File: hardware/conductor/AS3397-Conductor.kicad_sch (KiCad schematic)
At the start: 37 parts, among them J1 ES, J11 POWER, J2 AudioJack3, J2 MIDI IN, Q1 BS170F, U1 TL072, U4 Teensy-LC, U5 6N138

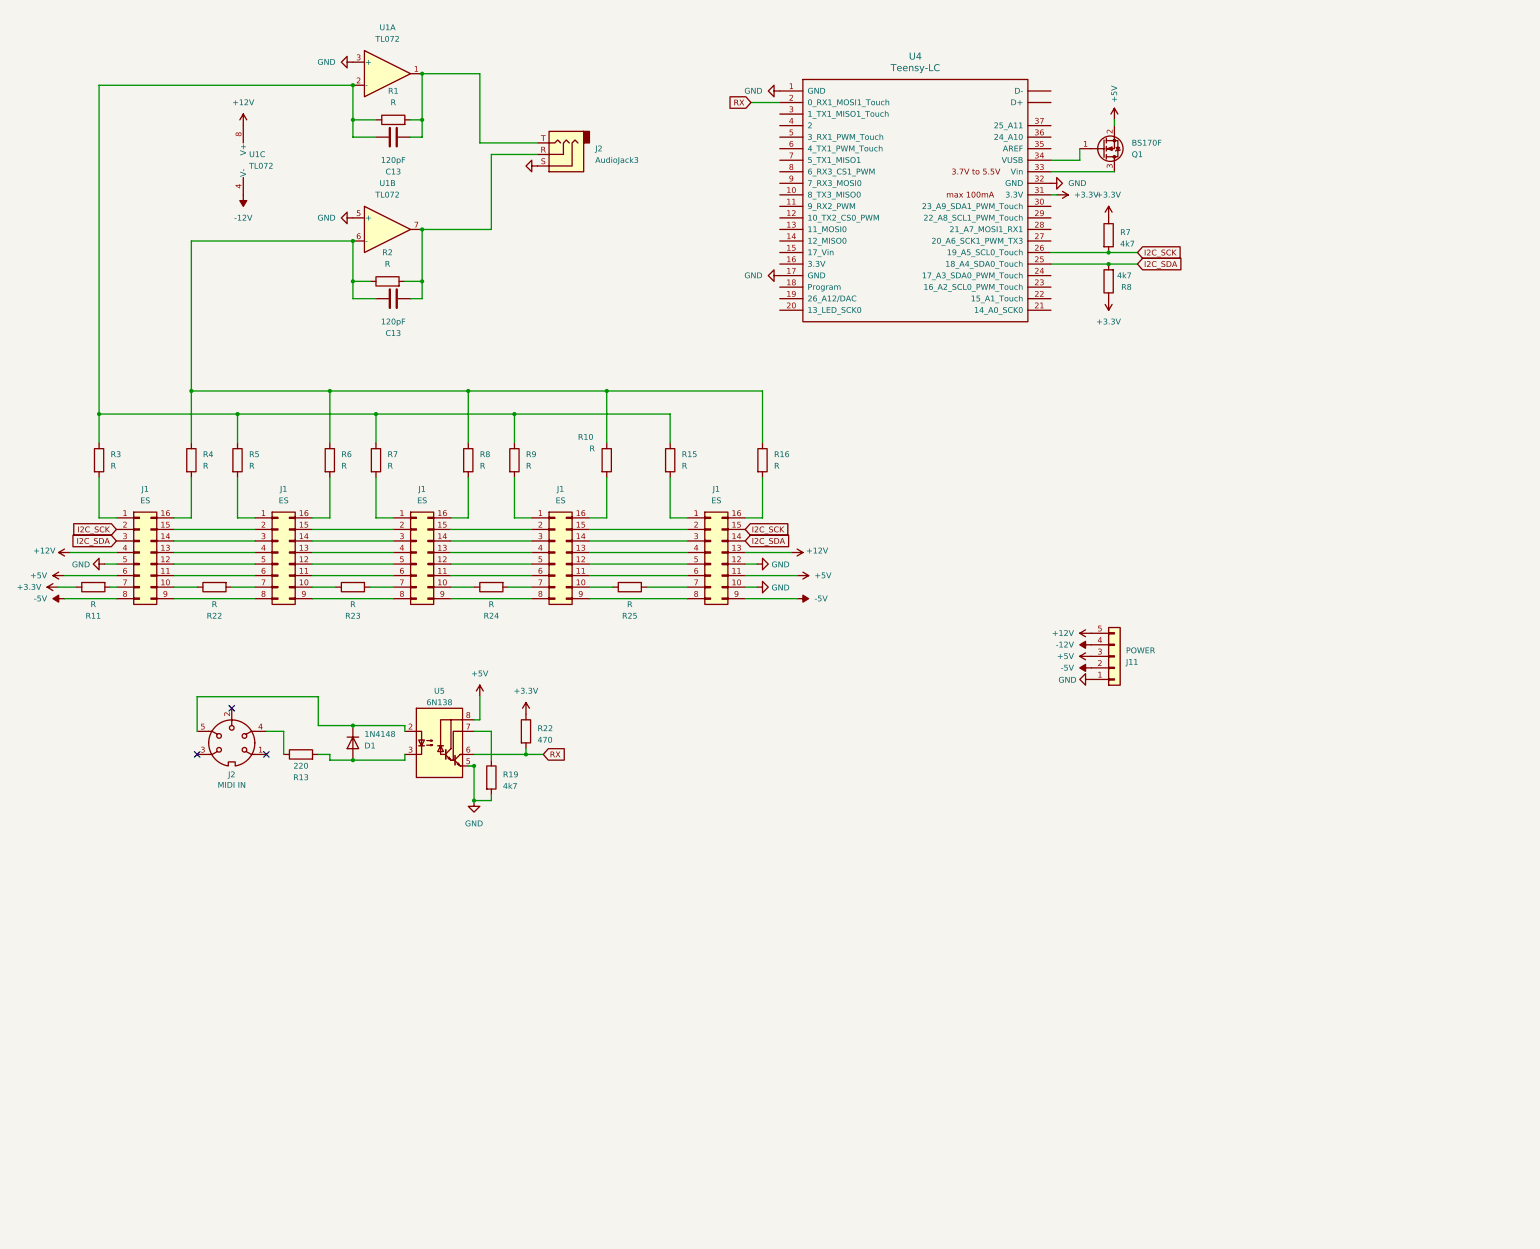
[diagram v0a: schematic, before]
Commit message: Conductor board new version
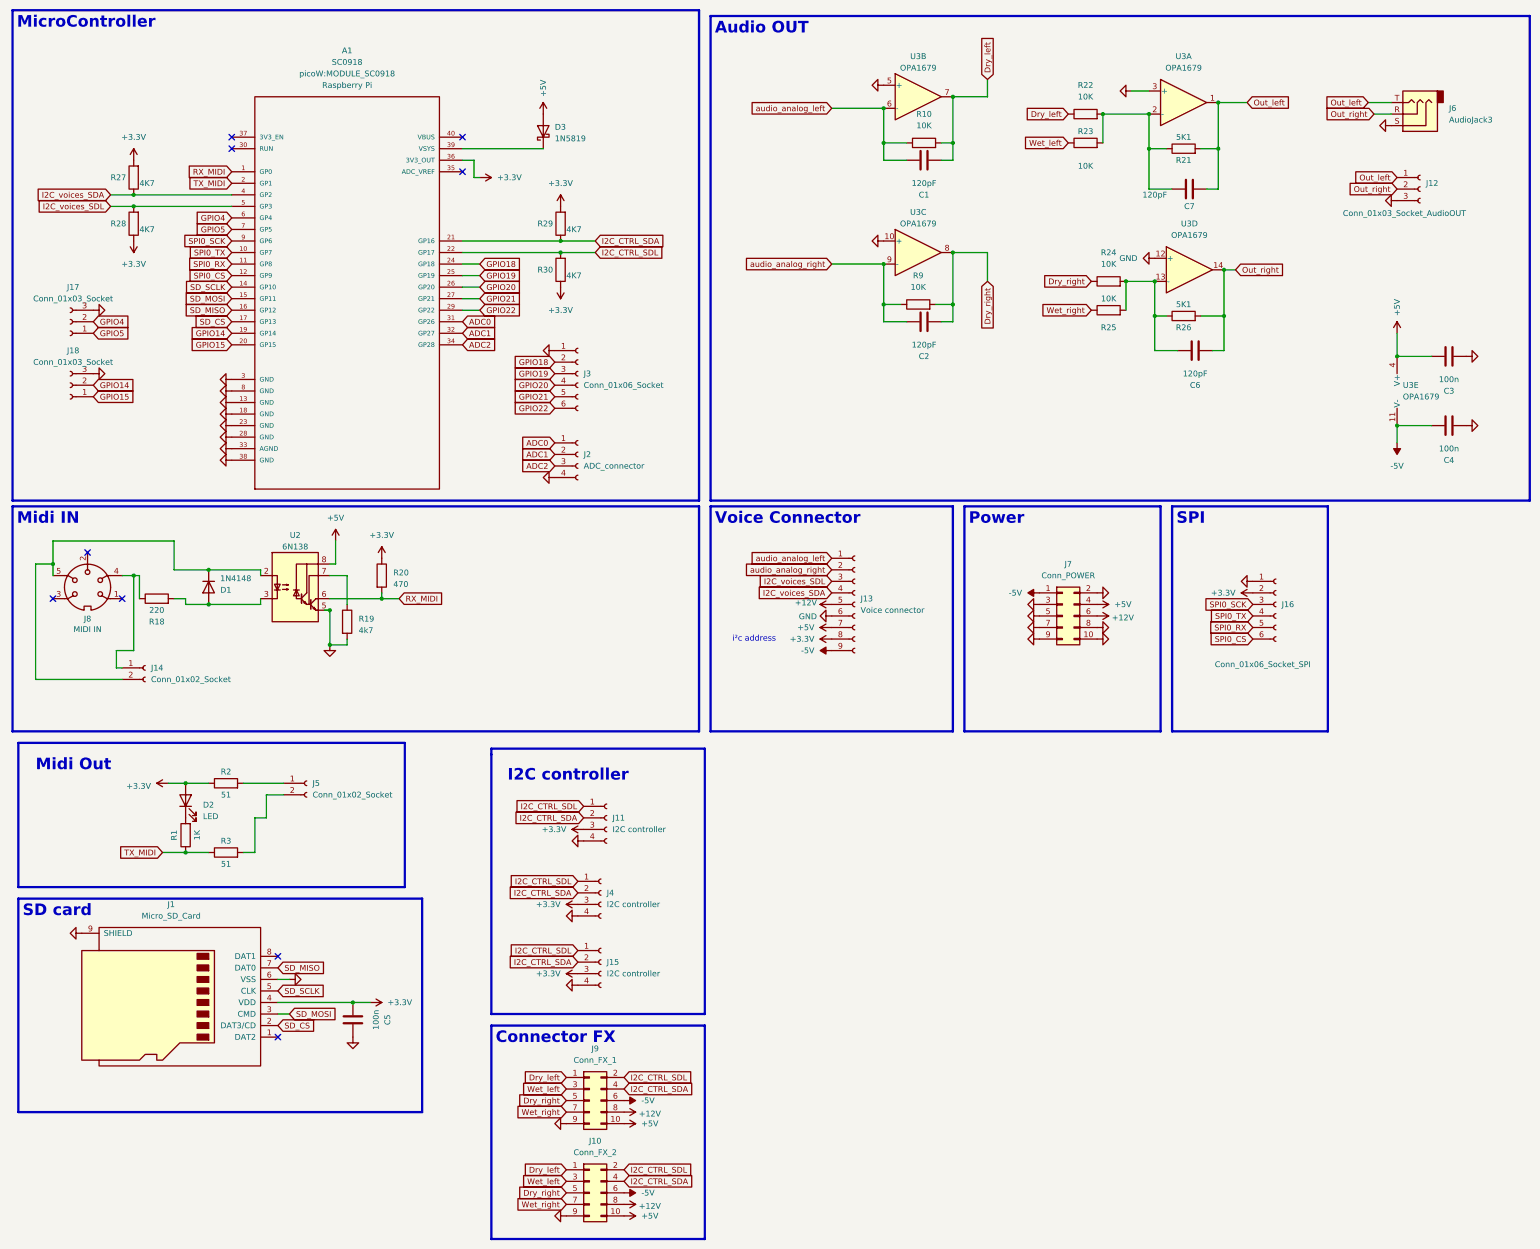
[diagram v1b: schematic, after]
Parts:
- removed C13 (x2): 120pF, Capacitor_THT:C_Disc_D4.3mm_W1.9mm_P5.00mm, symbol Device:C
- removed J1 (x5): ES, SYNTHFILLE:DIP-16_AS, symbol Connector_Generic:Conn_02x08_Counter_Clockwise
- removed J11: POWER, TerminalBlock:TerminalBlock_bornier-4_P5.08mm, symbol Connector_Generic:Conn_01x05
- removed J2: AudioJack3, Connector_Audio:Jack_3.5mm_Ledino_KB3SPRS_Horizontal, symbol Connector_Audio:AudioJack3
- removed J2: MIDI IN, lib:MIDI_DIN5, symbol ES1-rescue:DIN-5-MIDI
- removed Q1: BS170F, Package_TO_SOT_SMD:SOT-23, symbol Transistor_FET:BS170F
- removed R1, R11, R15, R16, R2, R22, R3, R4, R5, R6, R7, R8: R, Resistor_THT:R_Axial_DIN0204_L3.6mm_D1.6mm_P7.62mm_Horizontal, symbol Device:R
- removed R13: 220, Resistor_THT:R_Axial_DIN0204_L3.6mm_D1.6mm_P7.62mm_Horizontal, symbol Device:R
- removed R22: 470, Resistor_THT:R_Axial_DIN0204_L3.6mm_D1.6mm_P7.62mm_Horizontal, symbol Device:R
- removed R7, R8: 4k7, Resistor_THT:R_Axial_DIN0204_L3.6mm_D1.6mm_P7.62mm_Horizontal, symbol Device:R
- removed U1: TL072, Package_DIP:DIP-8_W7.62mm_LongPads, symbol Amplifier_Operational:TL072
- removed U4: Teensy-LC, symbol teensy:Teensy-LC
- removed U5: 6N138, Package_DIP:DIP-8_W7.62mm_LongPads, symbol Isolator:6N138
- added A1: SC0918, picoW:MODULE_SC0918, symbol Raspberry_Pi_Pico_W_SC0918:SC0918
- added C1, C2, C6, C7: 120pF, Capacitor_SMD:C_1206_3216Metric_Pad1.33x1.80mm_HandSolder, symbol Device:C
- added C3, C4, C5: 100n, Capacitor_SMD:C_1206_3216Metric_Pad1.33x1.80mm_HandSolder, symbol Device:C
- added D2: LED, Diode_THT:D_A-405_P2.54mm_Vertical_AnodeUp, symbol Device:LED
- added D3: 1N5819, Diode_THT:D_DO-41_SOD81_P10.16mm_Horizontal, symbol Diode:1N5819
- added J1: Micro_SD_Card, SD_card:J_SD_Card-micro_socket_A, symbol Connector:Micro_SD_Card
- added J10: Conn_FX_2, Connector_PinHeader_2.54mm:PinHeader_2x05_P2.54mm_Vertical, symbol Connector_Generic:Conn_02x05_Odd_Even
- added J11, J15, J4: I2C controller, Connector_JST:JST_EH_B4B-EH-A_1x04_P2.50mm_Vertical, symbol Connector:Conn_01x04_Socket
- added J12: Conn_01x03_Socket_AudioOUT, Connector_JST:JST_EH_B3B-EH-A_1x03_P2.50mm_Vertical, symbol Connector:Conn_01x03_Socket
- added J13: Voice connector, Connector_JST:JST_EH_B9B-EH-A_1x09_P2.50mm_Vertical, symbol Connector:Conn_01x09_Socket
- added J14, J5: Conn_01x02_Socket, Connector_JST:JST_EH_B2B-EH-A_1x02_P2.50mm_Vertical, symbol Connector:Conn_01x02_Socket
- added J16: Conn_01x06_Socket_SPI, Connector_PinSocket_2.54mm:PinSocket_1x06_P2.54mm_Vertical, symbol Connector:Conn_01x06_Socket
- added J17, J18: Conn_01x03_Socket, Connector_PinHeader_2.54mm:PinHeader_1x03_P2.54mm_Vertical, symbol Connector:Conn_01x03_Socket
- added J2: ADC_connector, Connector_JST:JST_EH_B4B-EH-A_1x04_P2.50mm_Vertical, symbol Connector:Conn_01x04_Socket
- added J3: Conn_01x06_Socket, Connector_PinHeader_2.54mm:PinHeader_1x06_P2.54mm_Vertical, symbol Connector:Conn_01x06_Socket
- added J6: AudioJack3, Connector_Audio:Jack_3.5mm_Ledino_KB3SPRS_Horizontal, symbol Connector_Audio:AudioJack3
- added J7: Conn_POWER, Connector_PinHeader_2.54mm:PinHeader_2x05_P2.54mm_Vertical, symbol Connector_Generic:Conn_02x05_Odd_Even
- added J8: MIDI IN, Eurocad:MIDI_DIN5, symbol ES1-rescue:DIN-5-MIDI
- added J9: Conn_FX_1, Connector_PinHeader_2.54mm:PinHeader_2x05_P2.54mm_Vertical, symbol Connector_Generic:Conn_02x05_Odd_Even
- added R1: 1K, Resistor_SMD:R_1206_3216Metric_Pad1.30x1.75mm_HandSolder, symbol Audio_chip:R
- added R18: 220, Resistor_SMD:R_1206_3216Metric_Pad1.30x1.75mm_HandSolder, symbol Device:R
- added R2, R3: 51, Resistor_SMD:R_1206_3216Metric_Pad1.30x1.75mm_HandSolder, symbol Audio_chip:R
- added R20: 470, Resistor_SMD:R_1206_3216Metric_Pad1.30x1.75mm_HandSolder, symbol Device:R
- added R21, R26: 5K1, Resistor_SMD:R_1206_3216Metric_Pad1.30x1.75mm_HandSolder, symbol Device:R
- added R22: 10K, Resistor_SMD:R_1206_3216Metric_Pad1.30x1.75mm_HandSolder, symbol Device:R
- added R27, R28, R29, R30: 4K7, Resistor_SMD:R_1206_3216Metric_Pad1.30x1.75mm_HandSolder, symbol Device:R
- added U2: 6N138, Package_DIP:DIP-8_W7.62mm_LongPads, symbol Isolator:6N138
- added U3: OPA1679, Package_SO:SOIC-14_3.9x8.7mm_P1.27mm, symbol Amplifier_Operational:TL074
- R10, R23, R24, R25, R9: value R -> 10K; footprint Resistor_THT:R_Axial_DIN0204_L3.6mm_D1.6mm_P7.62mm_Horizontal -> Resistor_SMD:R_1206_3216Metric_Pad1.30x1.75mm_HandSolder
- R19: footprint Resistor_THT:R_Axial_DIN0204_L3.6mm_D1.6mm_P7.62mm_Horizontal -> Resistor_SMD:R_1206_3216Metric_Pad1.30x1.75mm_HandSolder
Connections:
- net +12V: now also J10.8 (Pin_8), J13.5 (Pin_5), J7.6 (Pin_6), J9.8 (Pin_8)
- net +3.3V: now also A1.36 (3V3_OUT), C5.2, D2.2 (A), J1.4 (VDD), J11.3 (Pin_3), J13.8 (Pin_8), J15.3 (Pin_3), J16.2 (Pin_2), J4.3 (Pin_3), R2.1, R20.1, R27.2, R28.1, R29.2, R30.1
- net +5V: now also C3.1, D3.2 (A), J10.10 (Pin_10), J13.7 (Pin_7), J7.4 (Pin_4), J9.10 (Pin_10), U2.8 (VCC), U3.4 (V+)
- net -5V: now also C4.1, J10.6 (Pin_6), J13.9 (Pin_9), J7.1 (Pin_1), J9.6 (Pin_6), U3.11 (V-)
- net GND: now also A1.13 (GND), A1.18 (GND), A1.23 (GND), A1.28 (GND), A1.3 (GND), A1.33 (AGND), A1.38 (GND), A1.8 (GND), C3.2, C4.2, C5.1, J1.6 (VSS), J1.9 (SHIELD), J10.9 (Pin_9), J11.4 (Pin_4), J12.3 (Pin_3), J13.6 (Pin_6), J15.4 (Pin_4), J16.1 (Pin_1), J17.3 (Pin_3), J18.3 (Pin_3), J2.4 (Pin_4), J3.1 (Pin_1), J4.4 (Pin_4), J6.S, J7.10 (Pin_10), J7.2 (Pin_2), J7.3 (Pin_3), J7.5 (Pin_5), J7.7 (Pin_7), J7.8 (Pin_8), J7.9 (Pin_9), J9.9 (Pin_9), U2.5 (GND), U3.10 (+), U3.12 (+), U3.3 (+), U3.5 (+)
- net at R19.1: now also U2.7 (VO1)
- net Dry_right: now reaches R24.1
- net Dry_right: now also R9.2, C2.2, J10.5 (Pin_5), J9.5 (Pin_5), U3.8
- net at R23.2: now also C7.1, R21.1, R22.2, U3.2 (-)
- net audio_analog_left: now reaches R10.1
- net audio_analog_left: now also C1.1, J13.1 (Pin_1), U3.6 (-)
- net audio_analog_right: now reaches R9.1
- net audio_analog_right: now also C2.1, J13.2 (Pin_2), U3.9 (-)
- net at D1.1 (K): now also J14.2 (Pin_2), J8.5, U2.2 (C1)
- net at D1.2 (A): now also R18.2, U2.3 (C2)
- net Wet_left: now reaches R23.1
- net Wet_left: now also J10.3 (Pin_3), J9.3 (Pin_3)
- net Wet_right: now reaches R25.1
- net Wet_right: now also J10.7 (Pin_7), J9.7 (Pin_7)
- net at R25.2: now also R24.2, C6.1, R26.1, U3.13 (-)
- net Dry_left: now reaches R10.2
- net Dry_left: now also C1.2, J10.1 (Pin_1), J9.1 (Pin_1), R22.1, U3.7
- new net: J14.1 (Pin_1), J8.4, R18.1
- new net: A1.39 (VSYS), D3.1 (K)
- new net: D2.1 (K), R1.2
- new net: J5.2 (Pin_2), R3.2
- new net: J5.1 (Pin_1), R2.2
- new net ADC0: A1.31 (GP26), J2.1 (Pin_1)
- new net ADC1: A1.32 (GP27), J2.2 (Pin_2)
- new net ADC2: A1.34 (GP28), J2.3 (Pin_3)
- new net GPIO14: A1.19 (GP14), J18.2 (Pin_2)
- new net GPIO15: A1.20 (GP15), J18.1 (Pin_1)
- new net GPIO18: A1.24 (GP18), J3.2 (Pin_2)
- new net GPIO19: A1.25 (GP19), J3.3 (Pin_3)
- new net GPIO20: A1.26 (GP20), J3.4 (Pin_4)
- new net GPIO21: A1.27 (GP21), J3.5 (Pin_5)
- new net GPIO22: A1.29 (GP22), J3.6 (Pin_6)
- new net GPIO4: A1.6 (GP4), J17.2 (Pin_2)
- new net GPIO5: A1.7 (GP5), J17.1 (Pin_1)
- new net I2C_CTRL_SDA: A1.21 (GP16), J10.4 (Pin_4), J11.2 (Pin_2), J15.2 (Pin_2), J4.2 (Pin_2), J9.4 (Pin_4), R29.1
- new net I2C_CTRL_SDL: A1.22 (GP17), J10.2 (Pin_2), J11.1 (Pin_1), J15.1 (Pin_1), J4.1 (Pin_1), J9.2 (Pin_2), R30.2
- new net I2C_voices_SDA: A1.4 (GP2), J13.4 (Pin_4), R27.1
- new net I2C_voices_SDL: A1.5 (GP3), J13.3 (Pin_3), R28.2
- new net Out_left: C7.2, J12.1 (Pin_1), J6.T, R21.2, U3.1
- new net Out_right: C6.2, J12.2 (Pin_2), J6.R, R26.2, U3.14
- new net RX_MIDI: A1.1 (GP0), R20.2, U2.6 (VO2)
- new net SD_CS: A1.17 (GP13), J1.2 (DAT3/CD)
- new net SD_MISO: A1.16 (GP12), J1.7 (DAT0)
- new net SD_MOSI: A1.15 (GP11), J1.3 (CMD)
- new net SD_SCLK: A1.14 (GP10), J1.5 (CLK)
- new net SPI0_CS: A1.12 (GP9), J16.6 (Pin_6)
- new net SPI0_RX: A1.11 (GP8), J16.5 (Pin_5)
- new net SPI0_SCK: A1.9 (GP6), J16.3 (Pin_3)
- new net SPI0_TX: A1.10 (GP7), J16.4 (Pin_4)
- new net TX_MIDI: A1.2 (GP1), R1.1, R3.1
- no-connect marks 3 -> 9
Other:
- note added: "I2C controller"
- note added: "Midi Out"
- note added: "i²c address"
